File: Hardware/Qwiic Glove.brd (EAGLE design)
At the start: 25.4 x 36.8 mm, 35 parts, among them U1 ADS1015, U4 LMV358

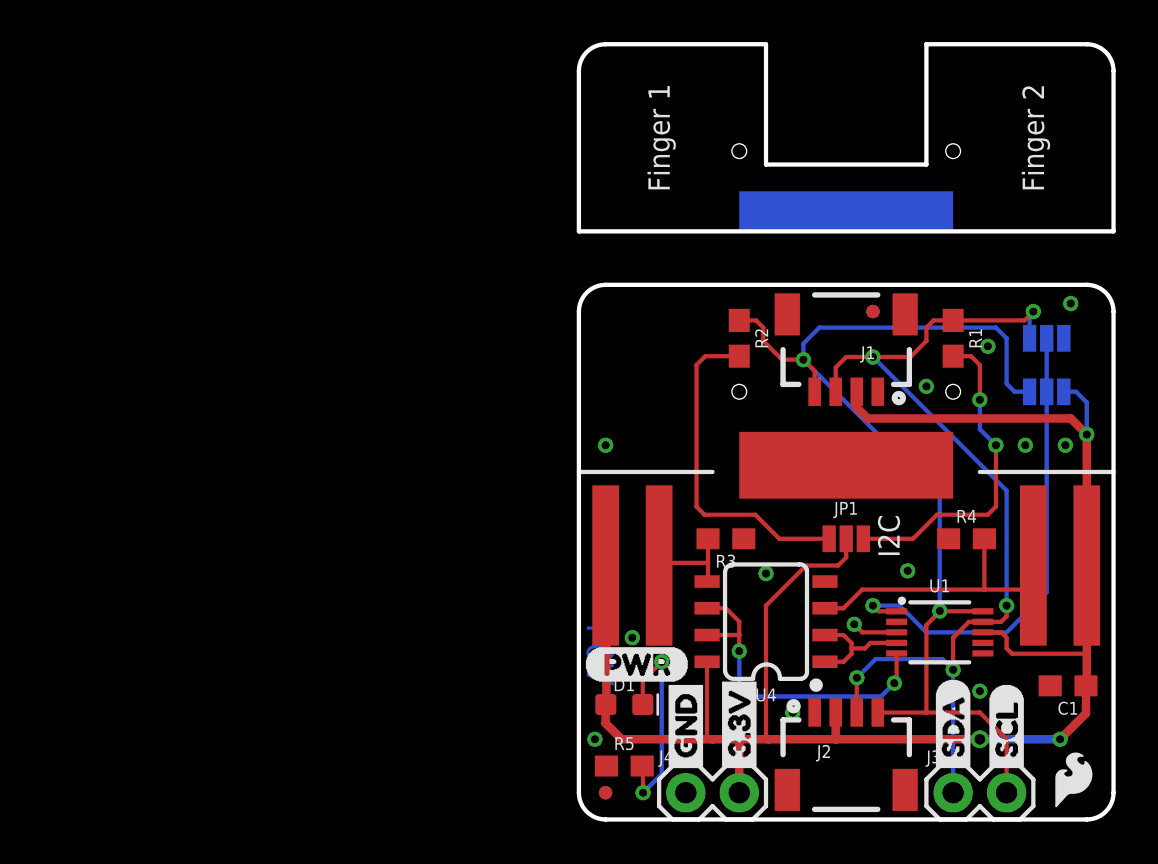
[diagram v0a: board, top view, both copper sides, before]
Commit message: post checklist changes
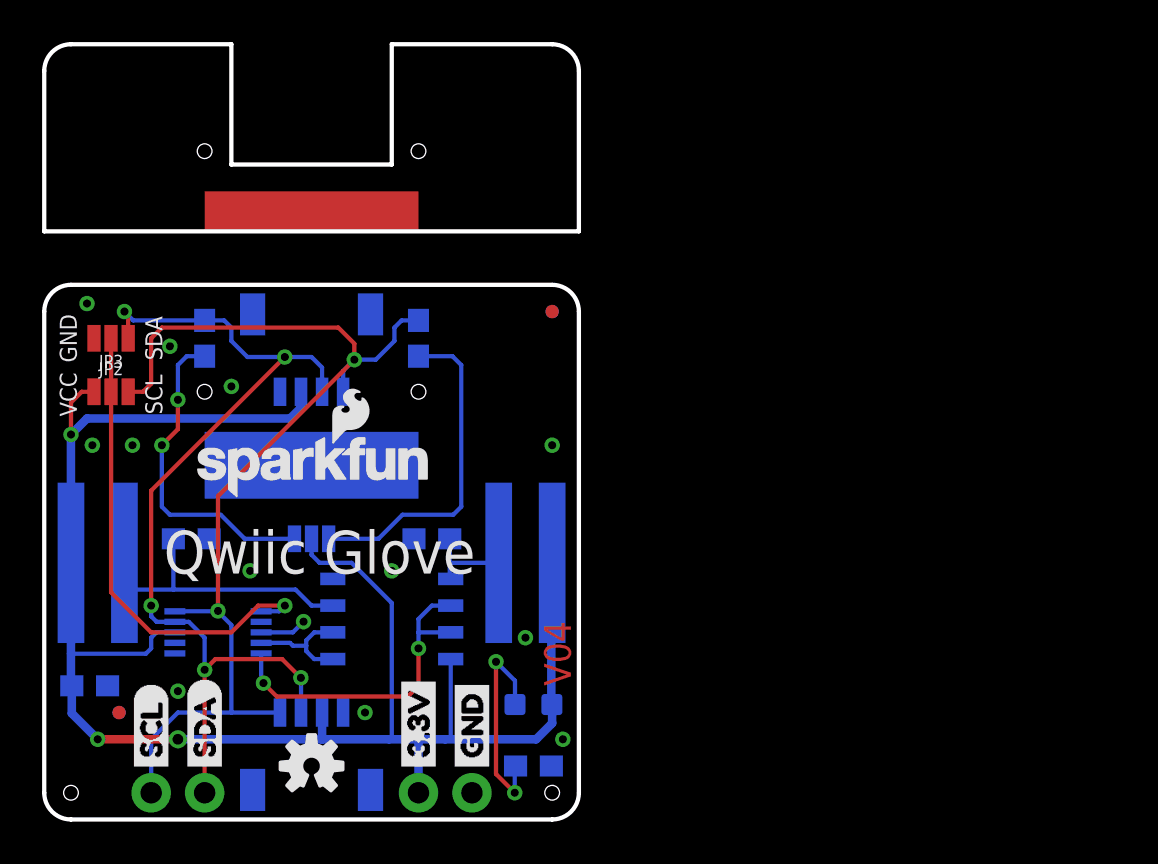
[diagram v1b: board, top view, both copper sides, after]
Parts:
- removed U$3, U$4: FLEX_SENSOR, Andy:FLEX_SENSOR
- added R6, R7: FLEX_SENSOR-4.5", SparkFun-Resistors:FLEX_SENSOR
- moved C1 46.5 mm to (-23.2, 6.35), flipped to the bottom
- moved JP2 44.5 mm to (-22.2, 22.9), flipped to the top
- moved JP3 44.5 mm to (-22.2, 20.3), flipped to the top
- moved LOGO3 44.2 mm to (-21.8, 0.38), flipped to the bottom
- moved U$10 40.6 mm to (-20.3, 2.03), flipped to the top
- moved U$9 40.6 mm to (-20.3, 2.03), flipped to the bottom
- moved LOGO1 37.1 mm to (-18.5, 15.2), flipped to the top
- moved R4 36.8 mm to (-18.4, 13.3), flipped to the bottom
- moved J3 35.6 mm to (-17.8, 1.27), flipped to the bottom
- moved R1 35.6 mm to (-17.8, 22.9), flipped to the bottom
- moved U$7 35.6 mm to (-17.8, 2.03), flipped to the bottom
- moved U$8 35.6 mm to (-17.8, 2.03), flipped to the top
- moved U1 34.3 mm to (-17.1, 8.89), flipped to the bottom
- moved J1 25.4 mm to (-12.7, 20.3), flipped to the bottom
- moved J2 25.4 mm to (-12.7, 5.08), flipped to the bottom
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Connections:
- net N$3: now also R7.P$1; no longer U$3.P$1
- net N$4: now also R6.P$1; no longer U$4.P$1
- net VCC: now also R6.P$2, R7.P$2; no longer U$3.P$2, U$4.P$2
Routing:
- net VCC: track 85.6 -> 86.2 mm
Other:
- board text added: "Units in Inches"

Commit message: post review changes
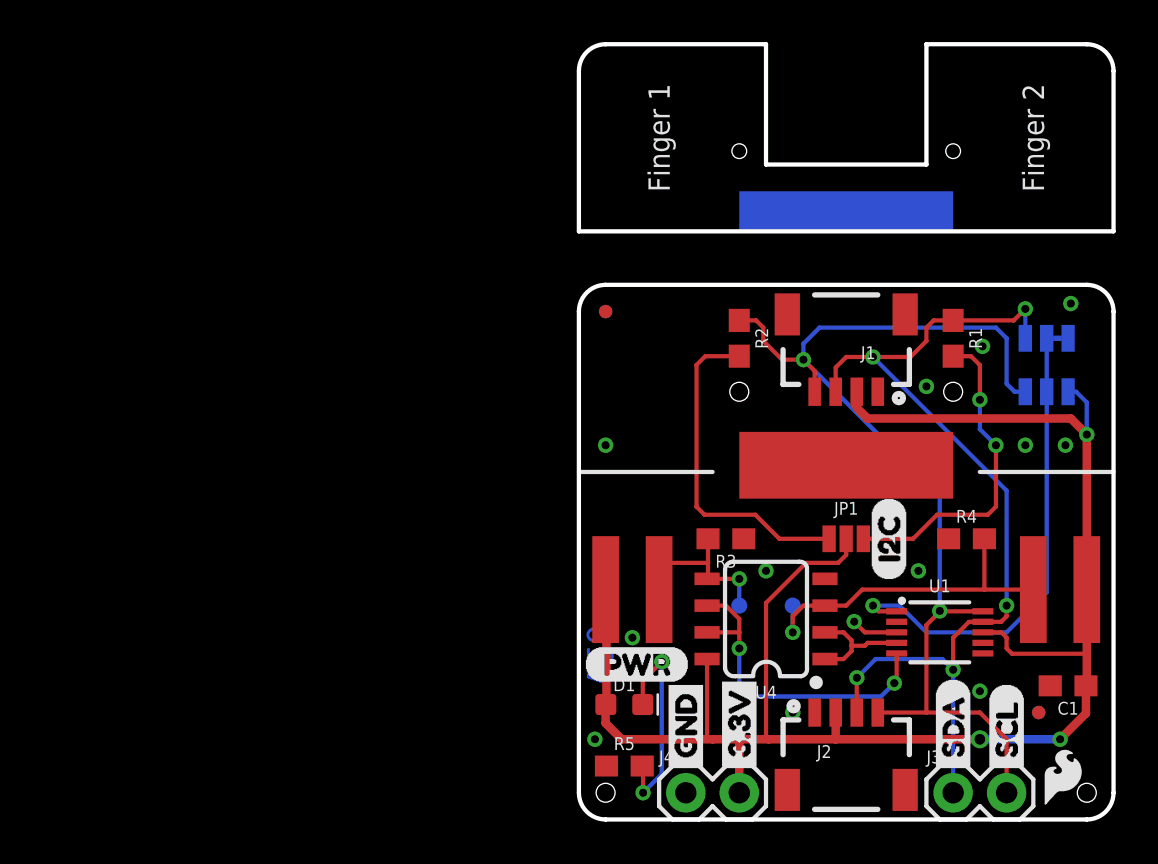
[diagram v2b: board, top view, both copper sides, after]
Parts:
- added TP1, TP2: TEST-POINT3, SparkFun-Connectors:PAD.03X.03
- added U$12: (no value), buzzard_labels (3):SDA0
- added U$13: (no value), buzzard_labels (4):SCL2
- added U$14: (no value), buzzard_labels (4):QWIIC_GLOVE1
- added U$15: (no value), Labels:I2C-()
- added U$3: (no value), Labels:3V3-TEXT
- added U$4: (no value), Labels:GND-TEXT-03
- JP2: value JUMPER-SMT_3_1-NC_PASTE_NO-SILK -> JUMPER-SMT_3_1-NC_TRACE_NO-SILK; device SparkFun-Jumpers:SMT-JUMPER_3_1-NC_PASTE_NO-SILK -> SparkFun-Jumpers:SMT-JUMPER_3_1-NC_TRACE_NO-SILK
- JP3: value JUMPER-SMT_3_NO_NO-SILK -> JUMPER-SMT_3_NO_NO_SILK; device SparkFun-Jumpers:SMT-JUMPER_3_NO_NO-SILK -> SparkFun-Jumpers:SMT-JUMPER_3_0-NO_TRACE_NO-SILK
- moved C1 46.5 mm to (23.2, 6.35), flipped to the top
- moved R6 45.7 mm to (22.9, 12.2), flipped to the top
- moved JP2 44.5 mm to (22.2, 22.9), flipped to the bottom
- moved JP3 44.5 mm to (22.2, 20.3), flipped to the bottom
- moved FD1 43.7 mm to (21.8, 5.08), flipped to the top
- moved FD2 43.7 mm to (21.8, 5.08), flipped to the bottom
- moved LOGO3 43.7 mm to (21.8, 0.38), flipped to the top
- moved U$10 40.6 mm to (20.3, 2.03), flipped to the bottom
- moved U$9 40.6 mm to (20.3, 2.03), flipped to the top
- moved LOGO1 37.1 mm to (18.5, 15.2), flipped to the bottom
- moved R4 36.8 mm to (18.4, 13.3), flipped to the top
- moved J3 35.6 mm to (17.8, 1.27), flipped to the top
- moved R1 35.6 mm to (17.8, 22.9), flipped to the top
- moved U$7 35.6 mm to (17.8, 2.03), flipped to the top
- moved U$8 35.6 mm to (17.8, 2.03), flipped to the bottom
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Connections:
- net N$3: now also R7.P$2, TP2.P$1; no longer R7.P$1
- net N$4: now also TP1.P$1
- net VCC: now also R7.P$1; no longer R7.P$2
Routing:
- net N$3: track 4.25 -> 8.32 mm, vias 0 -> 1
- net N$4: track 13.9 -> 16.4 mm, vias 0 -> 1
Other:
- board text added: "v10"
- board text removed: "GND"
- board text removed: "I2C"
- board text removed: "Qwiic Glove"
- board text removed: "SCL"
- board text removed: "SDA"
- board text removed: "V04"
- board text removed: "VCC"
